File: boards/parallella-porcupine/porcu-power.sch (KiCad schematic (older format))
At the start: 6 parts, among them J1 CONN\\HDR\\P1\\2R15, J11 CONN\\HDR\\2MM\\2R07\\SHD, J12 CONN\\HDR\\P1\\1R02, J13 CONN\\HDR\\P1\\1R02, J14 CONN\\HDR\\P1\\2R15

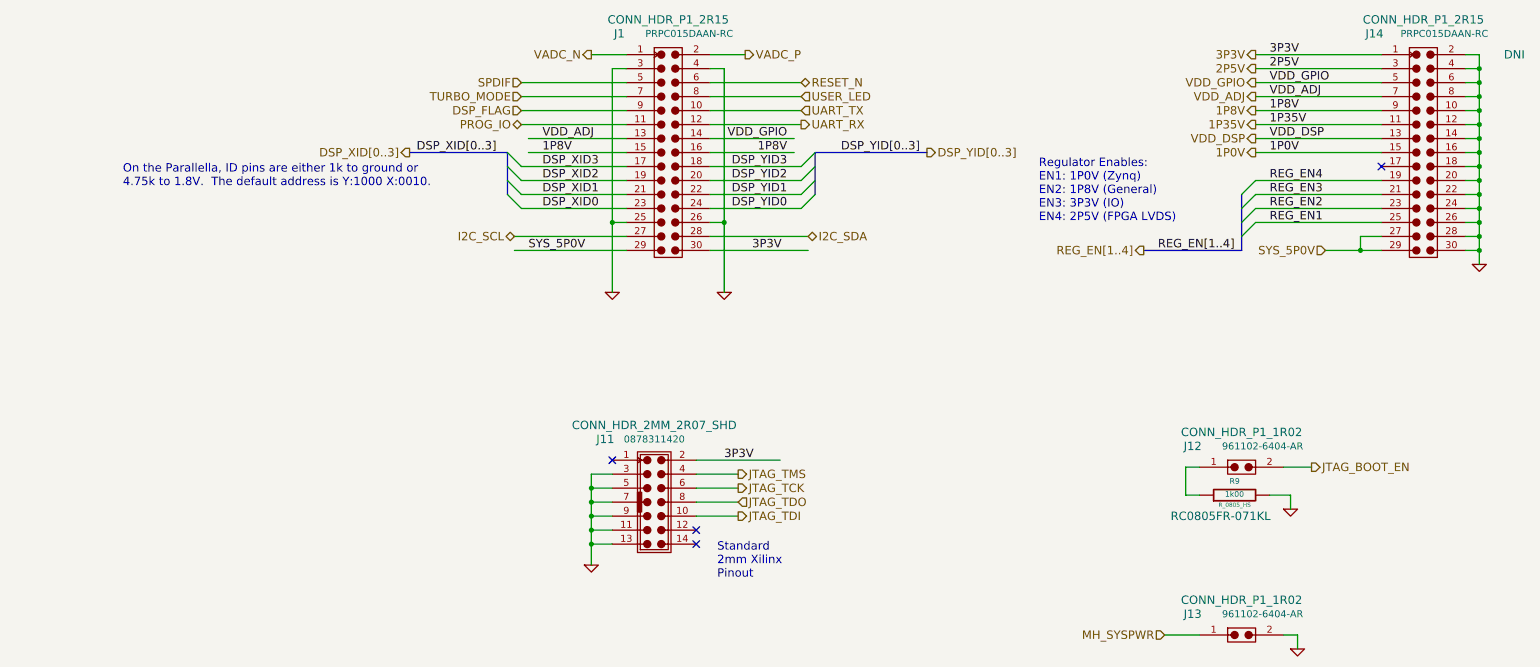
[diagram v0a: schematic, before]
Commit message: Ready for full review.
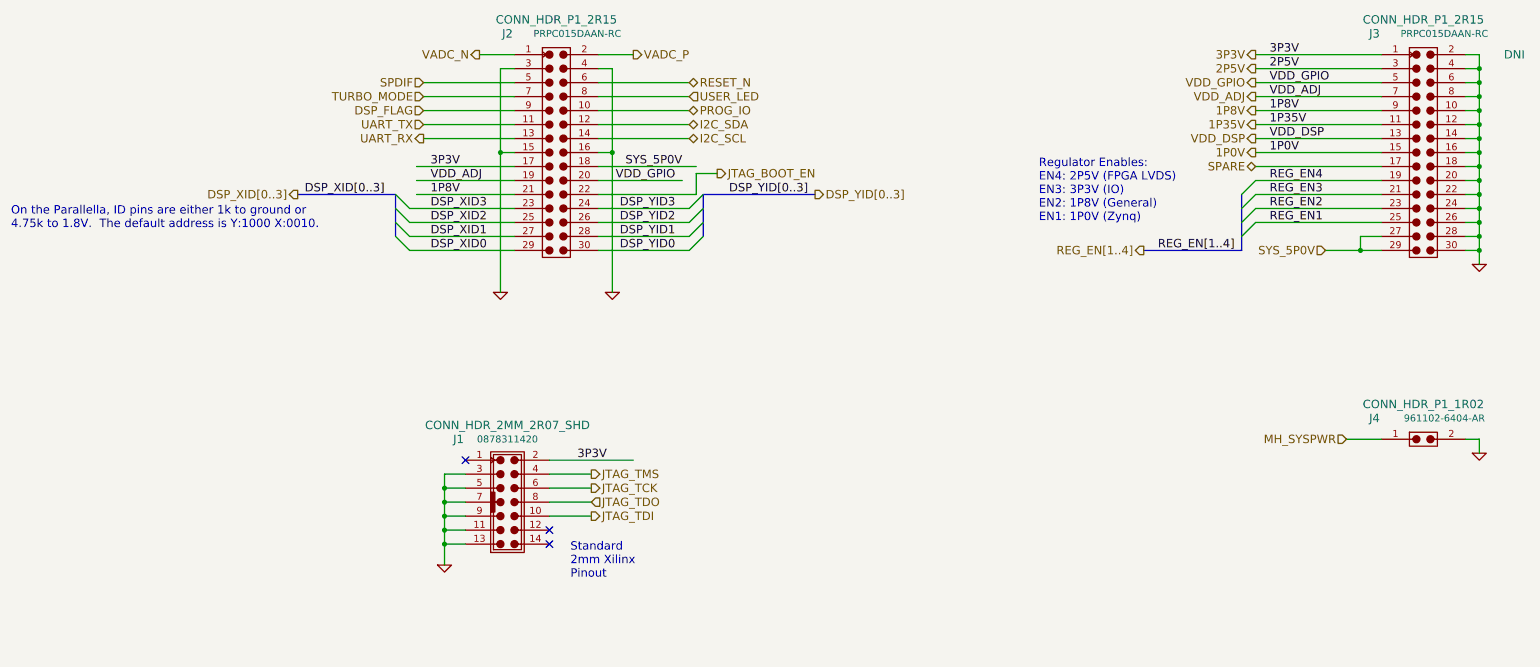
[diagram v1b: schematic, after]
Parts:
- removed J12: CONN\\HDR\\P1\\1R02, CONN_HDR_P1_1R02, symbol CONN\HDR\P1\1R02
- removed R9: 1k00, R_0805_HS, symbol R\SMD0805\1PCT\1K00
- renumbered J11 to J1, J1 to J2, J14 to J3, J13 to J4
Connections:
- net labels added: SPARE
- wire segments 84 -> 81
- no-connect marks 4 -> 3
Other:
- note added: "Regulator Enables:\nEN4: 2P5V (FPGA LVDS)\nEN3: 3P3V (IO)\nEN2: 1P8V (General)\nEN1: 1P0V (Zynq)"
- note removed: "Regulator Enables:\nEN1: 1P0V (Zynq)\nEN2: 1P8V (General)\nEN3: 3P3V (IO)\nEN4: 2P5V (FPGA LVDS)"
- moved on the sheet: J1, J2, J4

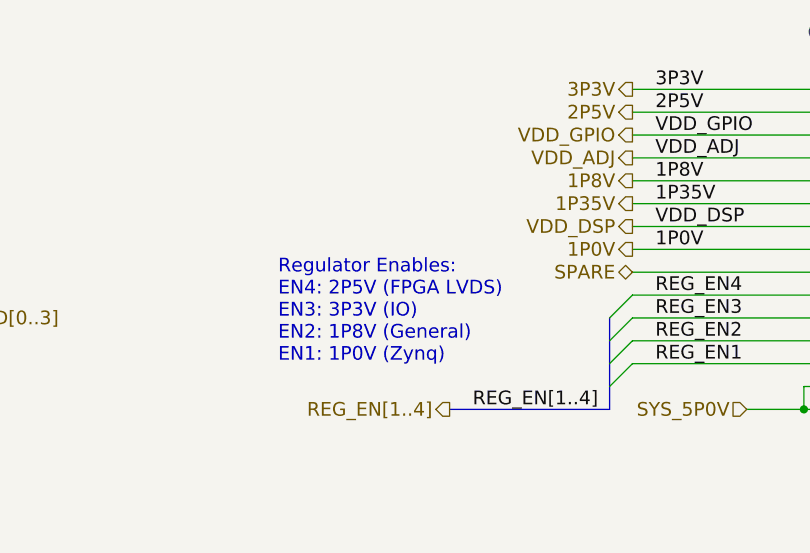
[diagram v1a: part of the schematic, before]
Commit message: Porcupine Version 2.
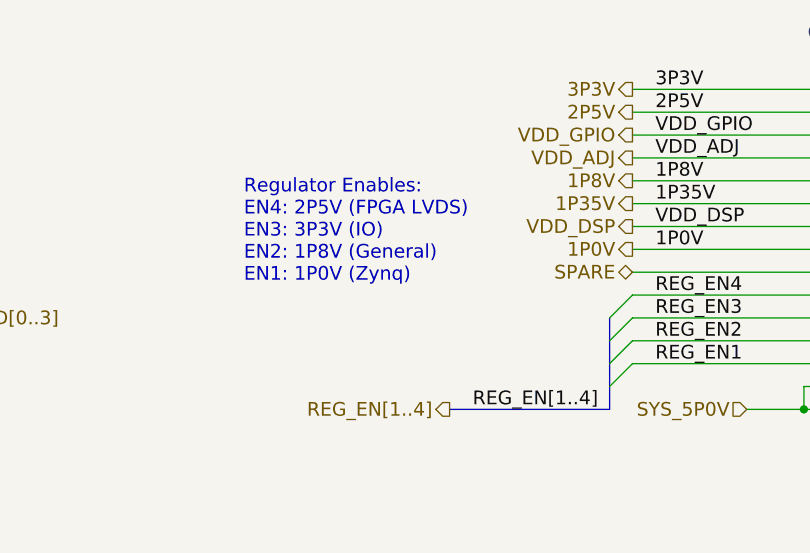
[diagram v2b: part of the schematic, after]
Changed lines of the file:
@@
 LIBS:valves
 LIBS:porcupine-cache
-EELAYER 24 0
+EELAYER 25 0
 EELAYER END
 $Descr B 17000 11000
 encoding utf-8
-Sheet 7 10
-Title "Parallella Breakout Daughtercard"
-Date "19 Jun 2014"
-Rev "*"
+Sheet 7 11
+Title "Parallella Breakout Daughtercard, Ver. 2"
+Date "17 feb 2015"
+Rev "A"
 Comp "Adapteva, Inc., 1666 Massachusetts Ave., Lexington, MA, 02420"
-Comment1 "including JTAG"
+Comment1 "Porcupine Top Level"
 Comment2 "Various Power connectors and Jumpers"
 Comment3 ""
@@
 Text Notes 2050 4400 0    60   ~ 0
 On the Parallella, ID pins are either 1k to ground or\n4.75k to 1.8V.  The default address is Y:1000 X:0010.
-Text Notes 9400 4350 0    60   ~ 0
+Text Notes 9250 4000 0    60   ~ 0
 Regulator Enables:\nEN4: 2P5V (FPGA LVDS)\nEN3: 3P3V (IO)\nEN2: 1P8V (General)\nEN1: 1P0V (Zynq)
 Entry Wire Line
